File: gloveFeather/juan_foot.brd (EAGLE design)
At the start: 40.6 x 58.1 mm, 9 parts

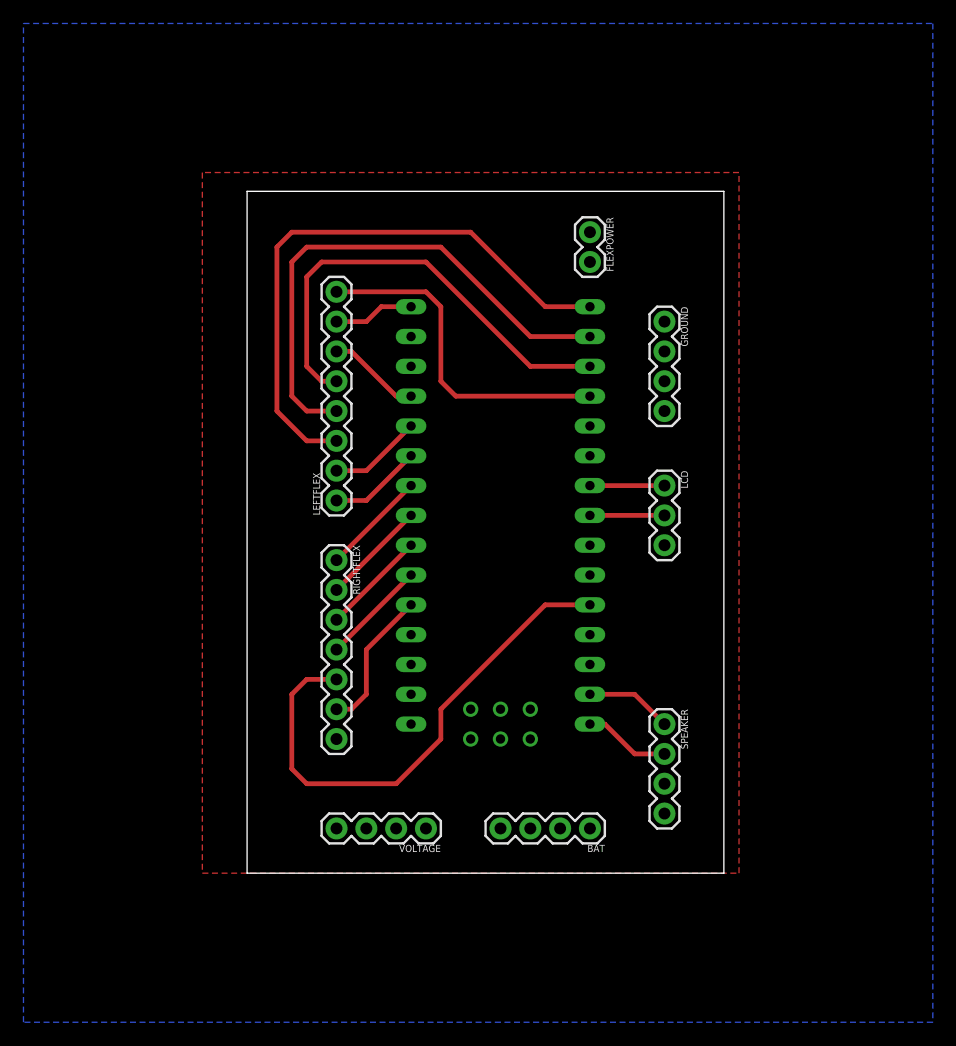
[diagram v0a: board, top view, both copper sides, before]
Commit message: final pcb
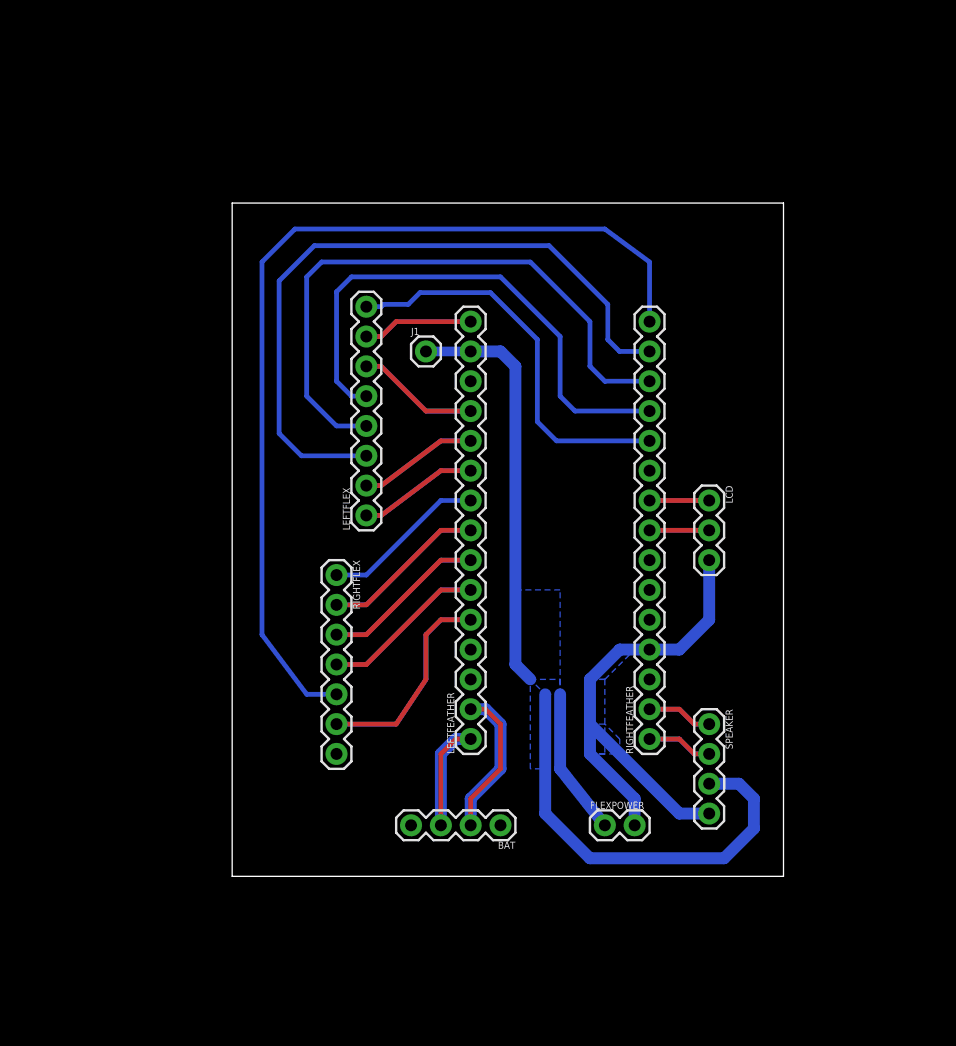
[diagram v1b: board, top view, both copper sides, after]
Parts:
- removed GROUND, VOLTAGE: (no value), SparkFun-Connectors:1X04
- removed U$1: NANO, Arduino-clone:NANO
- added J1: (no value), SparkFun-Connectors:1X01
- added LEFTFEATHER, RIGHTFEATHER: (no value), SparkFun-Connectors:1X15
- moved FLEXPOWER 50.5 mm to (31.8, 4.08), turned to 0 degrees
- moved BAT 7.62 mm to (22.9, 4.08)
- moved LCD 4.02 mm to (40.6, 31.8)
- moved SPEAKER 3.81 mm to (40.6, 12.7)
- moved LEFTFLEX 2.84 mm to (11.4, 30.5)
- moved RIGHTFLEX 1.27 mm to (8.89, 25.4)
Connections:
- removed net V: VOLTAGE.1, VOLTAGE.2, VOLTAGE.3, VOLTAGE.4
- new net 5V: LEFTFEATHER.4
- new net D3: RIGHTFEATHER.6
- new net D4: RIGHTFEATHER.7
- new net D7: RIGHTFEATHER.10
- new net N$13: LEFTFEATHER.13
- new net RST: LEFTFEATHER.3, RIGHTFEATHER.3
- new net VIN: BAT.3, LEFTFEATHER.1
- net 3V: now also J1.1, LEFTFEATHER.14; no longer BAT.3, U$1.RAW
- net GND: now also LEFTFEATHER.2, RIGHTFEATHER.4; no longer GROUND.1, GROUND.2, GROUND.3, GROUND.4, U$1.GND
- net INDEXFLEX: now also LEFTFEATHER.11; no longer U$1.A1
- net INDEXSIDE: now also LEFTFEATHER.9; no longer U$1.A3
- net INDEXTIP: now also RIGHTFEATHER.14; no longer U$1.D12
- net MIDDLEB: now also RIGHTFEATHER.12; no longer U$1.D10
- net MIDDLEFLEX: now also LEFTFEATHER.12; no longer U$1.A0
- net MIDDLESIDE: now also RIGHTFEATHER.13; no longer U$1.D11
- net MIDDLETIP: now also LEFTFEATHER.15; no longer U$1.D13
- net PINKYFLEX: now also LEFTFEATHER.5; no longer U$1.A7
- net PINKYSIDE: now also RIGHTFEATHER.15; no longer U$1.D2
- net RINGFLEX: now also LEFTFEATHER.6; no longer U$1.A6
- net RINGSIDE: now also RIGHTFEATHER.11; no longer U$1.D9
- net SCL: now also LEFTFEATHER.7; no longer U$1.A5
- net SDA: now also LEFTFEATHER.8; no longer U$1.A4
- net SIN: now also RIGHTFEATHER.2; no longer U$1.RX1
- net SOUT: now also RIGHTFEATHER.1; no longer U$1.TX0
- net SRX: now also RIGHTFEATHER.9; no longer U$1.D6
- net STX: now also RIGHTFEATHER.8; no longer U$1.D5
- net THUMBFLEX: now also LEFTFEATHER.10; no longer U$1.A2
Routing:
- net 3V: track 0.00 -> 85.3 mm
- net GND: track 0.00 -> 70.1 mm
- net PINKYSIDE: track 44.4 -> 80.8 mm
- net PINKYFLEX: track 12.3 -> 35.6 mm
- net SDA: track 8.98 -> 28.1 mm
- net SCL: track 8.98 -> 28.1 mm
- net RINGFLEX: track 8.98 -> 28.1 mm
- net VIN: track 0.00 -> 18.3 mm
- net MIDDLEFLEX: track 7.93 -> 20.9 mm
- net THUMBFLEX: track 7.93 -> 20.3 mm
- net INDEXFLEX: track 7.93 -> 20.3 mm
- net MIDDLETIP: track 6.88 -> 18.8 mm
- net INDEXTIP: track 49.9 -> 59.5 mm
- net MIDDLESIDE: track 44.8 -> 52.5 mm
- net MIDDLEB: track 39.0 -> 45.6 mm
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- added copper zone on layer 16, net 3V
- removed copper zone on layer 1, net 3V
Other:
- board size 40.6 x 58.1 mm -> 47 x 57.4 mm
